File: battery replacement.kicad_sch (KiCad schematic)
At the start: 15 parts, among them U1 GP3134_C48997205

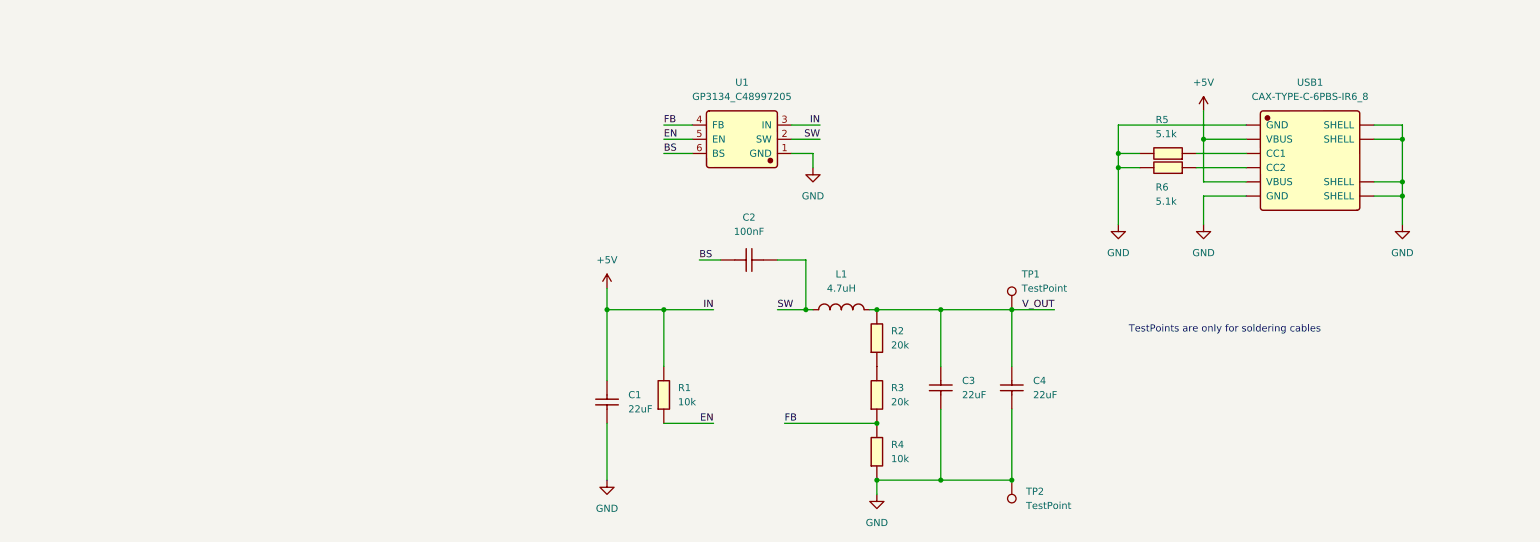
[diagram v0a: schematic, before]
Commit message: prelim. 10x25mm ~ 180pcs
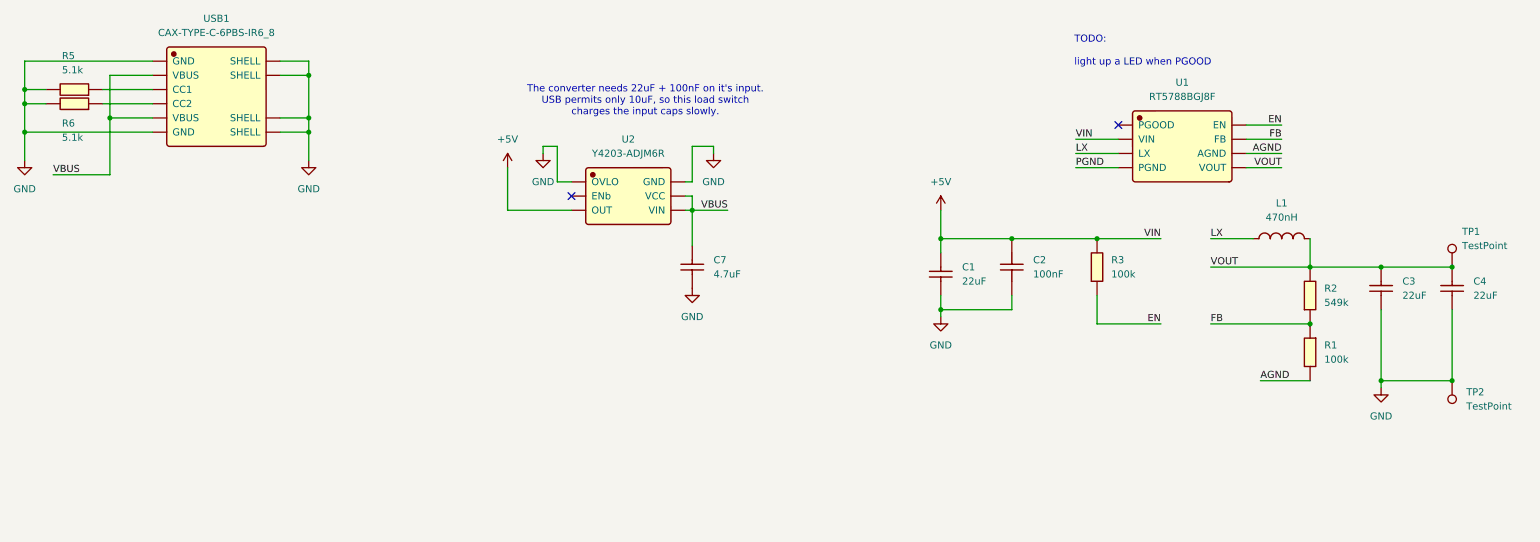
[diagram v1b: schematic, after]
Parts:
- removed L1: 4.7uH, JLCImport:BMQA000606304R7MA1, symbol JLCImport:BMQA000606304R7MA1
- removed R1, R4: 10k, JLCImport:0402WGF1002TCE, symbol JLCImport:0402WGF1002TCE
- removed R2, R3: 20k, JLCImport:0402WGF2002TCE, symbol JLCImport:0402WGF2002TCE
- removed U1: GP3134_C48997205, JLCImport:GP3134_C48997205, symbol JLCImport:GP3134_C48997205
- added C7: 4.7uF, JLCImport:CL21A475KAQNNNE, symbol JLCImport:CL21A475KAQNNNE
- added L1: 470nH, JLCImport:TMS252012ALM-R47MTAA, symbol JLCImport:TMS252012ALM-R47MTAA
- added R1, R3: 100k, JLCImport:0402WGF1003TCE, symbol JLCImport:0402WGF1003TCE
- added R2: 549k, JLCImport:0402WGF5493TCE, symbol JLCImport:0402WGF5493TCE
- added U1: RT5788BGJ8F, JLCImport:RT5788BGJ8F, symbol JLCImport:RT5788BGJ8F
- added U2: Y4203-ADJM6R, JLCImport:Y4203-ADJM6R, symbol JLCImport:Y4203-ADJM6R
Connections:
- net BS is gone; now on net GND: C2.2
- net SW is gone; now on net +5V: C2.1
- net +5V: now also C1.2, R3.2, U1.2 (VIN), U2.3 (OUT); no longer C1.1, USB1.A9 (VBUS), USB1.B9 (VBUS)
- net EN: now also R3.1, U1.8 (EN)
- net FB: now also R1.1, R2.1, U1.7 (FB)
- net GND: now also C1.1, C7.1, U2.1 (OVLO), U2.6 (GND); no longer C1.2
- net V_OUT renamed VOUT
- net VOUT: now also L1.2, R2.2, U1.5 (VOUT)
- new net AGND: R1.2, U1.6 (AGND)
- new net LX: L1.1, U1.3 (LX)
- new net PGND: U1.4 (PGND)
- new net VBUS: C7.2, U2.4 (VIN), U2.5 (VCC), USB1.A9 (VBUS), USB1.B9 (VBUS)
- no-connect marks 0 -> 2
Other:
- note added: "TODO: light up a LED when PGOOD"
- note added: "The converter needs 22uF + 100nF on it's input. USB permits only 10uF, so this load switch charges the input caps slowly."
- note removed: "TestPoints are only for soldering cables"
- moved on the sheet: C1, C2, C3, C4, R5, R6, TP1, TP2, USB1
